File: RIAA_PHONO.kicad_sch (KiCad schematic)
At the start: 21 parts, among them U1 OPA1644AxD, U2 OPA1612AxD

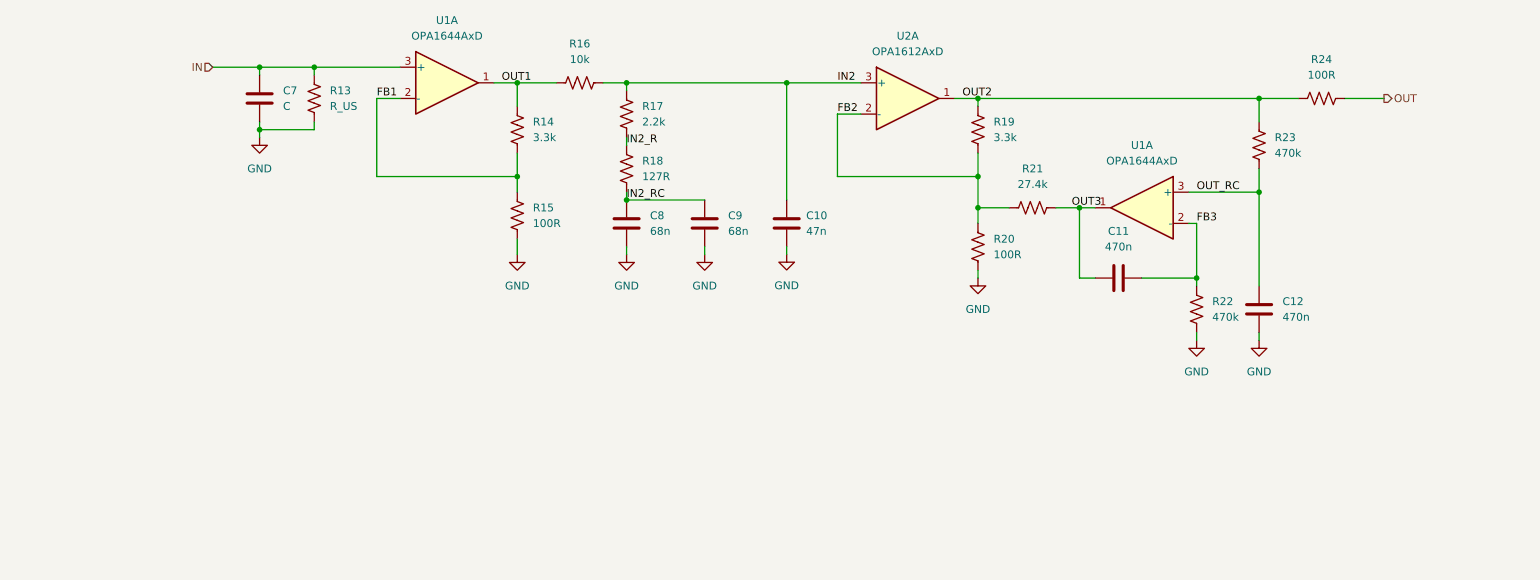
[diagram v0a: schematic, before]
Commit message: CHANGE POWER SUPPLY
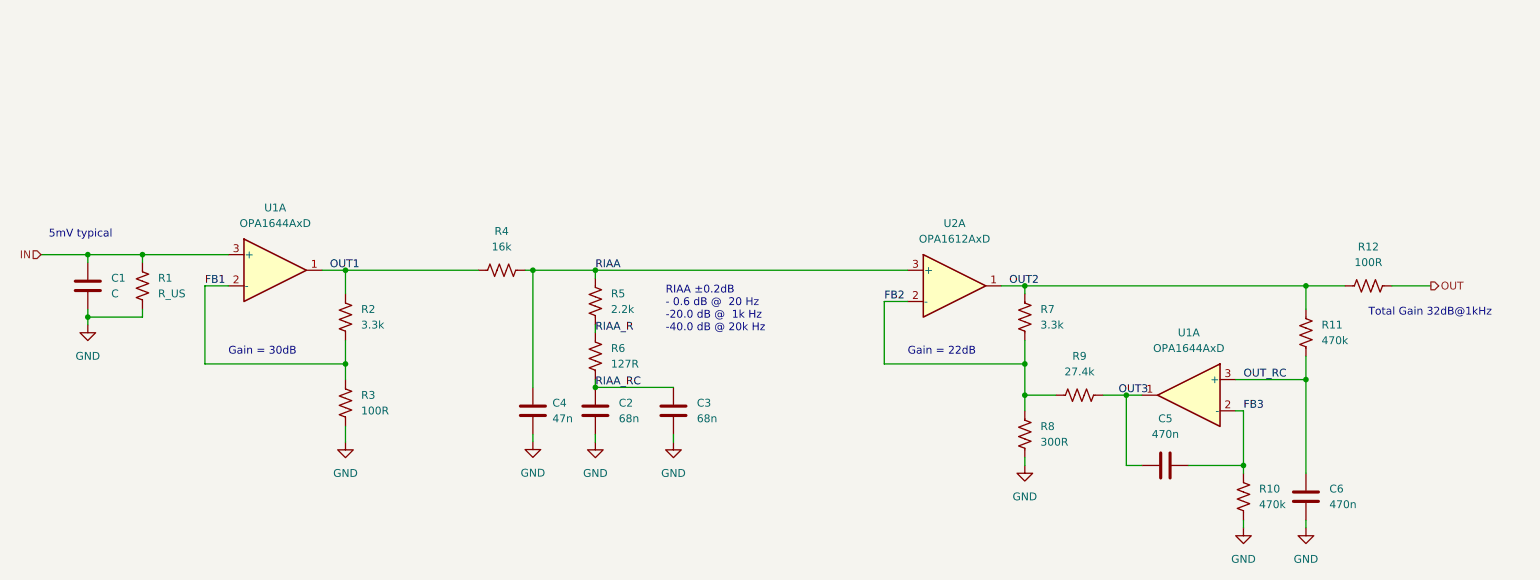
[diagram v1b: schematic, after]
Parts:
- R4: renamed from R16; value 10k -> 16k
- R8: renamed from R20; value 100R -> 300R
- renumbered C7 to C1, C8 to C2, C9 to C3, C10 to C4, C11 to C5, C12 to C6, R13 to R1, R22 to R10, R23 to R11, R24 to R12, R14 to R2, R15 to R3, R17 to R5, R18 to R6, R19 to R7, R21 to R9
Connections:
- net IN2 renamed RIAA
- net IN2_R renamed RIAA_R
- net IN2_RC renamed RIAA_RC
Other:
- note added: "5mV typical"
- note added: "Gain = 22dB"
- note added: "Gain = 30dB"
- note added: "RIAA ±0.2dB - 0.6 dB @ 20 Hz -20.0 dB @ 1k Hz -40.0 dB @ 20k Hz"
- note added: "Total Gain 32dB@1kHz"
- moved on the sheet: C1, C2, C3, C4, C5, C6, R1, R10, R11, R12, R2, R3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
